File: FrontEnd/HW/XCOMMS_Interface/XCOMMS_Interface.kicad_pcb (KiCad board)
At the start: 4 copper layers, 40 x 65 mm, 113 parts, among them J1 TFC-110-02-F-D-A-P-FR, J2 PicoBlade01x05, J3 PicoBlade01x05, J4 PicoBlade01x02, U1 STM32L431KBUx, U10 MAX870EUK, U11 STM32L053R8Tx, U2 TPS56637, U3 TPS56637, U4 TPS56637, U5 TPS784, U6 MAX870EUK, U7 INA290, U8 AD5160, U9 MAX870EUK, Y1 ECS-.327-7-34QCS-TR

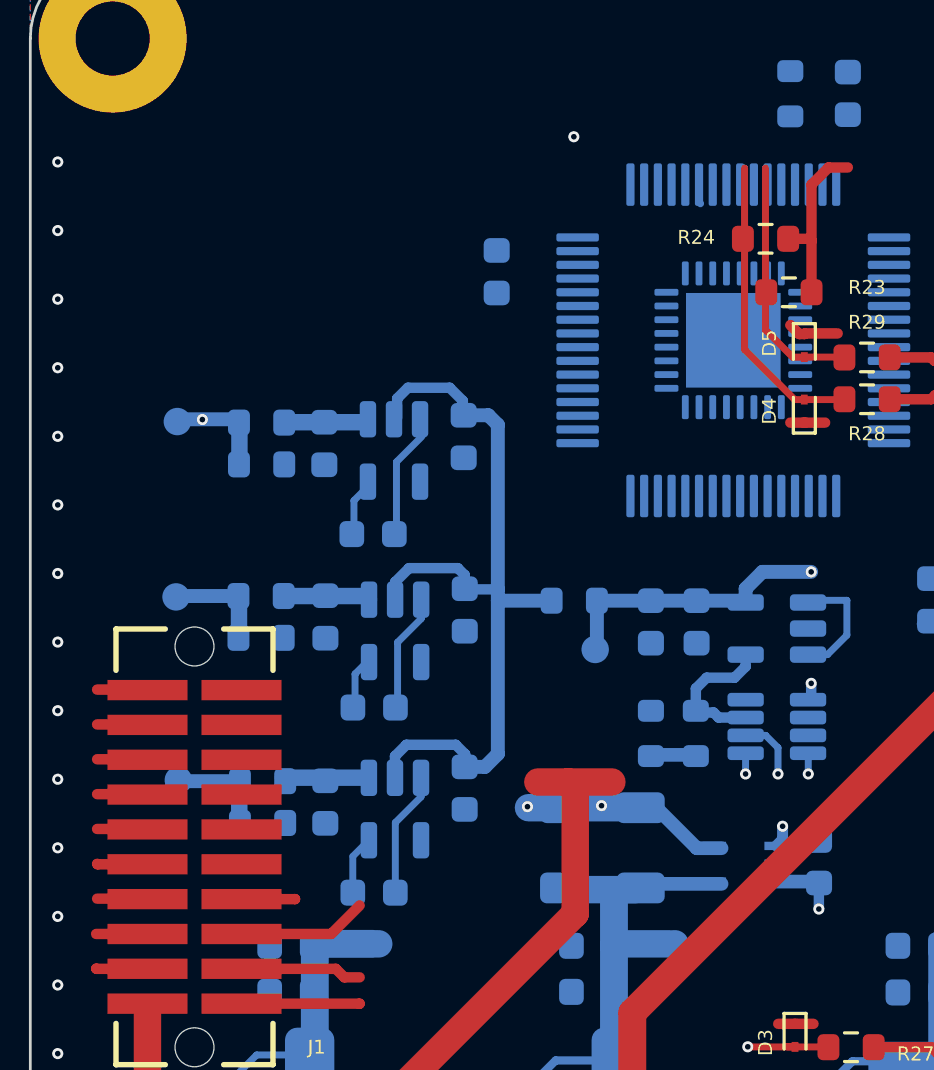
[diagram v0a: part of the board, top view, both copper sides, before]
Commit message: continuation of previous
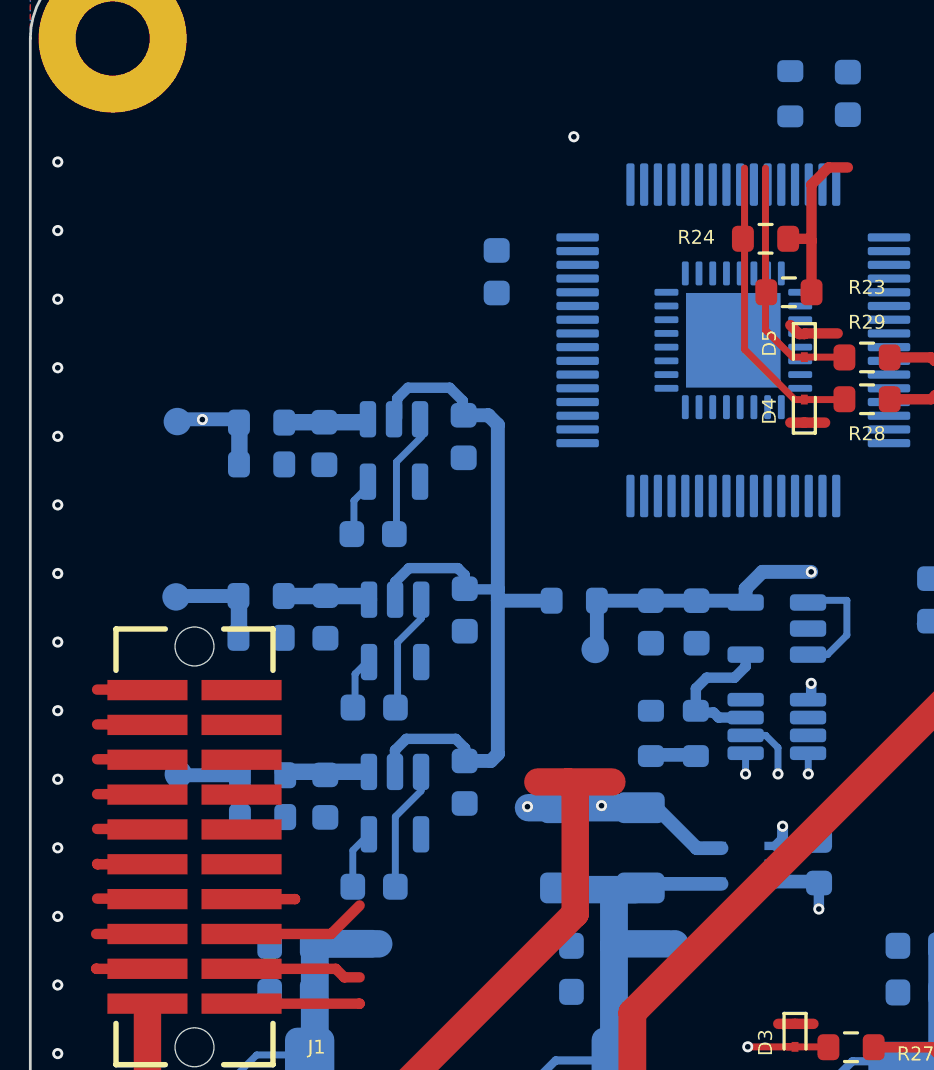
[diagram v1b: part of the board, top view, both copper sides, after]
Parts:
- moved TP7 0.22 mm to (133.4, 101.8)
- moved C38 0.22 mm to (138.8, 102.6)
- moved C39 0.22 mm to (143.8, 102.1)
- moved C40 0.22 mm to (140.5, 105.9)
- moved R20 0.22 mm to (136.5, 101.9)
- moved R21 0.22 mm to (136.5, 103.4)
- moved U10 0.22 mm to (141.3, 102.9)
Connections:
- U1 pad 10: unconnected-(U1-Pad10) -> /R_CSB
- U1 pad 19: unconnected-(U1-Pad19) -> /I2C1_SCL
- U1 pad 2: /RCC_IN -> unconnected-(U1-Pad2)
- U1 pad 20: unconnected-(U1-Pad20) -> /I2C1_SDA
- U1 pad 29: /I2C1_SCL -> unconnected-(U1-Pad29)
- U1 pad 3: /RCC_OUT -> unconnected-(U1-Pad3)
- U1 pad 30: /I2C1_SDA -> unconnected-(U1-Pad30)
- U1 pad 6: unconnected-(U1-Pad6) -> /RCC_IN_HSE
- U1 pad 9: /R_CSB -> unconnected-(U1-Pad9)
- U11 pad 17: /R_CSB -> unconnected-(U11-Pad17)
- U11 pad 20: unconnected-(U11-Pad20) -> /R_CSB
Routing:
- net +12V: track 109.4 -> 122.2 mm, vias 3 -> 5
- net +3V3: track 35.8 -> 27.5 mm, vias 1 -> 0
- net /NRST: track 7.73 -> 3.24 mm, vias 2 -> 1
- net /I2C1_SDA: track 10.5 -> 9.19 mm
- net /PLL_CSB: track 3.15 -> 1.84 mm
